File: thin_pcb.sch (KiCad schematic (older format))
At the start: 127 parts, among them J01 Conn_01x02, J02 Conn_01x02, J04 Conn_01x02, J06 Conn_01x02, J07 Conn_01x02, J08 Conn_01x02, J1 USB_B_Micro, J11 Conn_01x03, J12 Conn_01x03, J13 Conn_01x03, J14 Conn_01x03, J15 Conn_01x03, J16 Conn_01x03, J17 Conn_01x03, J18 Conn_01x03, J2 AudioJack4_Ground, J21 Conn_01x07, J22 Conn_01x07, J23 Conn_01x07, J24 Conn_01x07, J25 Conn_01x07, J26 Conn_01x07, J27 Conn_01x07, J28 Conn_01x07, J3 AudioJack4_Ground, J31 Conn_01x07, J32 Conn_01x07, J33 Conn_01x07, J34 Conn_01x07, J35 Conn_01x07, J36 Conn_01x07, J37 Conn_01x07, J38 Conn_01x07, J4 Conn_01x06, J41 Conn_01x04, J42 Conn_01x04, J43 Conn_01x04, J44 Conn_01x04, J45 Conn_01x04, J46 Conn_01x04, J47 Conn_01x04, J48 Conn_01x04, J5 Conn_01x06, J51 Conn_01x01, J52 Conn_01x01, J53 Conn_01x01, J54 Conn_01x01, J55 Conn_01x01, J56 Conn_01x01, J57 Conn_01x01, J58 Conn_01x01, J6 Conn_02x02, J7 Conn_01x02, SW11 SW_Push, SW12 SW_Push, SW13 SW_Push, SW14 SW_Push, SW15 SW_Push, SW21 SW_Push, SW22 SW_Push, SW23 SW_Push, SW24 SW_Push, SW25 SW_Push, SW252 SW_Push, SW31 SW_Push, SW32 SW_Push, SW33 SW_Push, SW34 SW_Push, SW35 SW_Push, SW41 SW_Push, SW42 SW_Push, SW422 SW_Push, SW43 SW_Push, SW44 SW_Push, SW45 SW_Push, SW452 SW_Push, SW51 SW_Push, SW52 SW_Push, SW522 SW_Push, SW53 SW_Push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

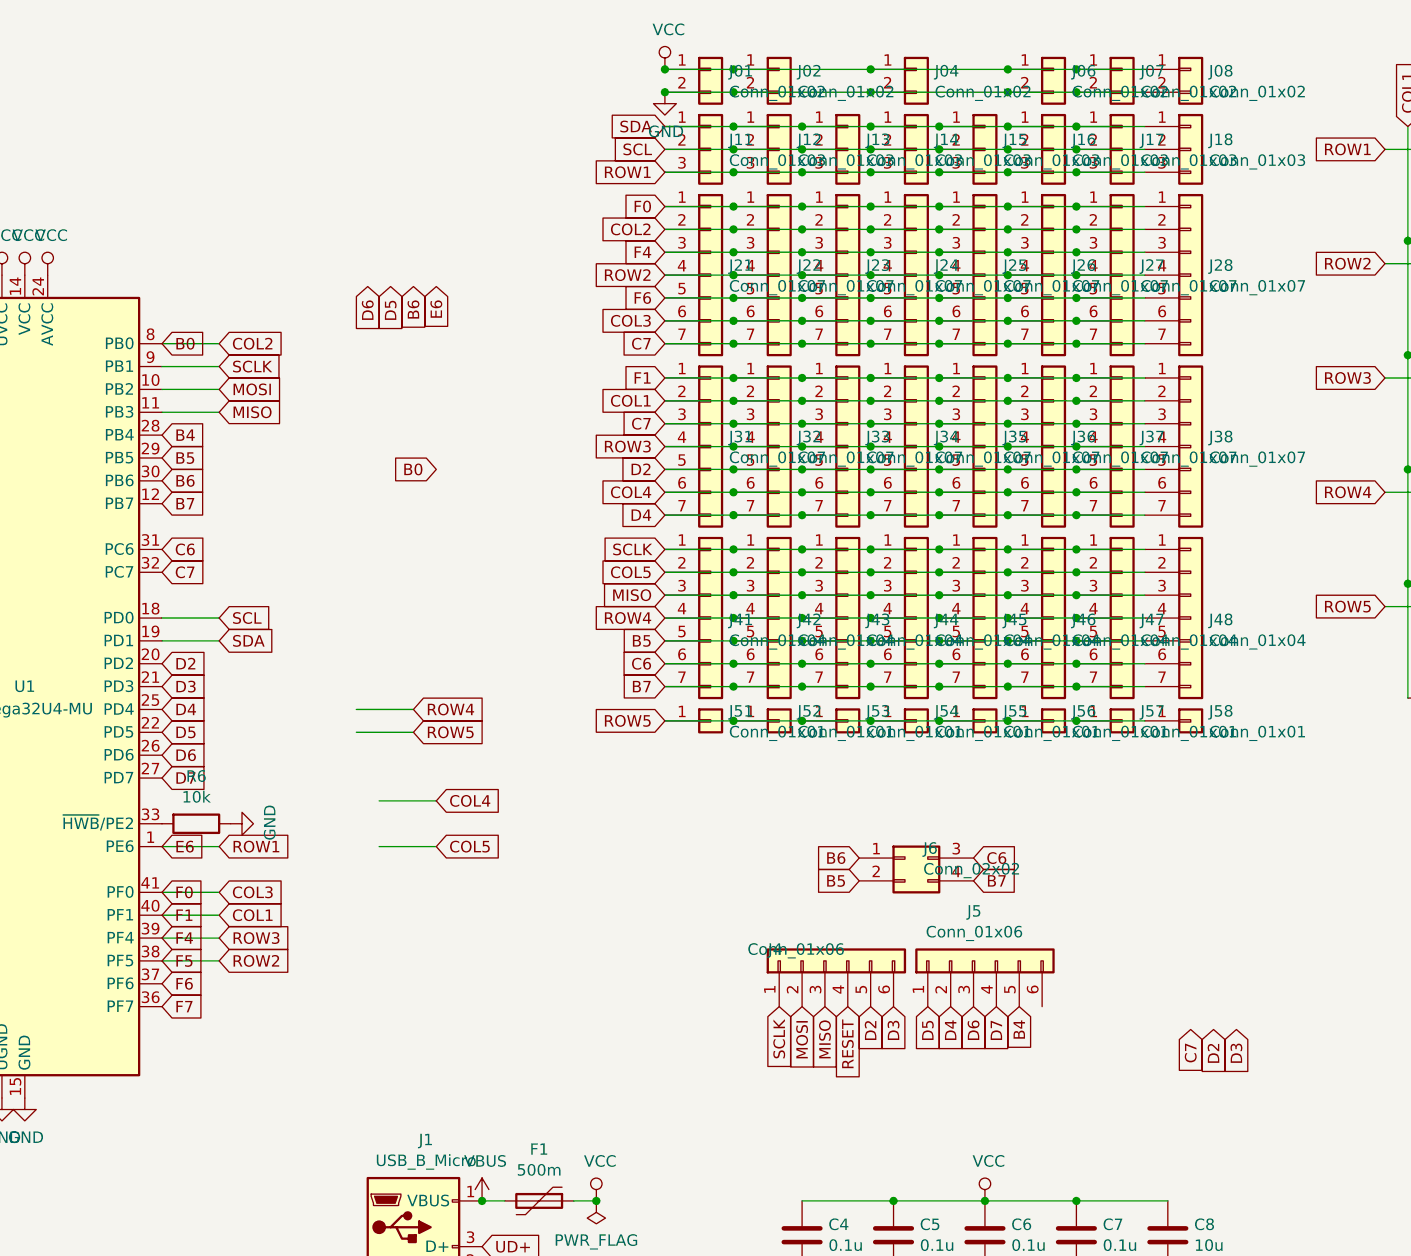
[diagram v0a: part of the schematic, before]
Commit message: draft
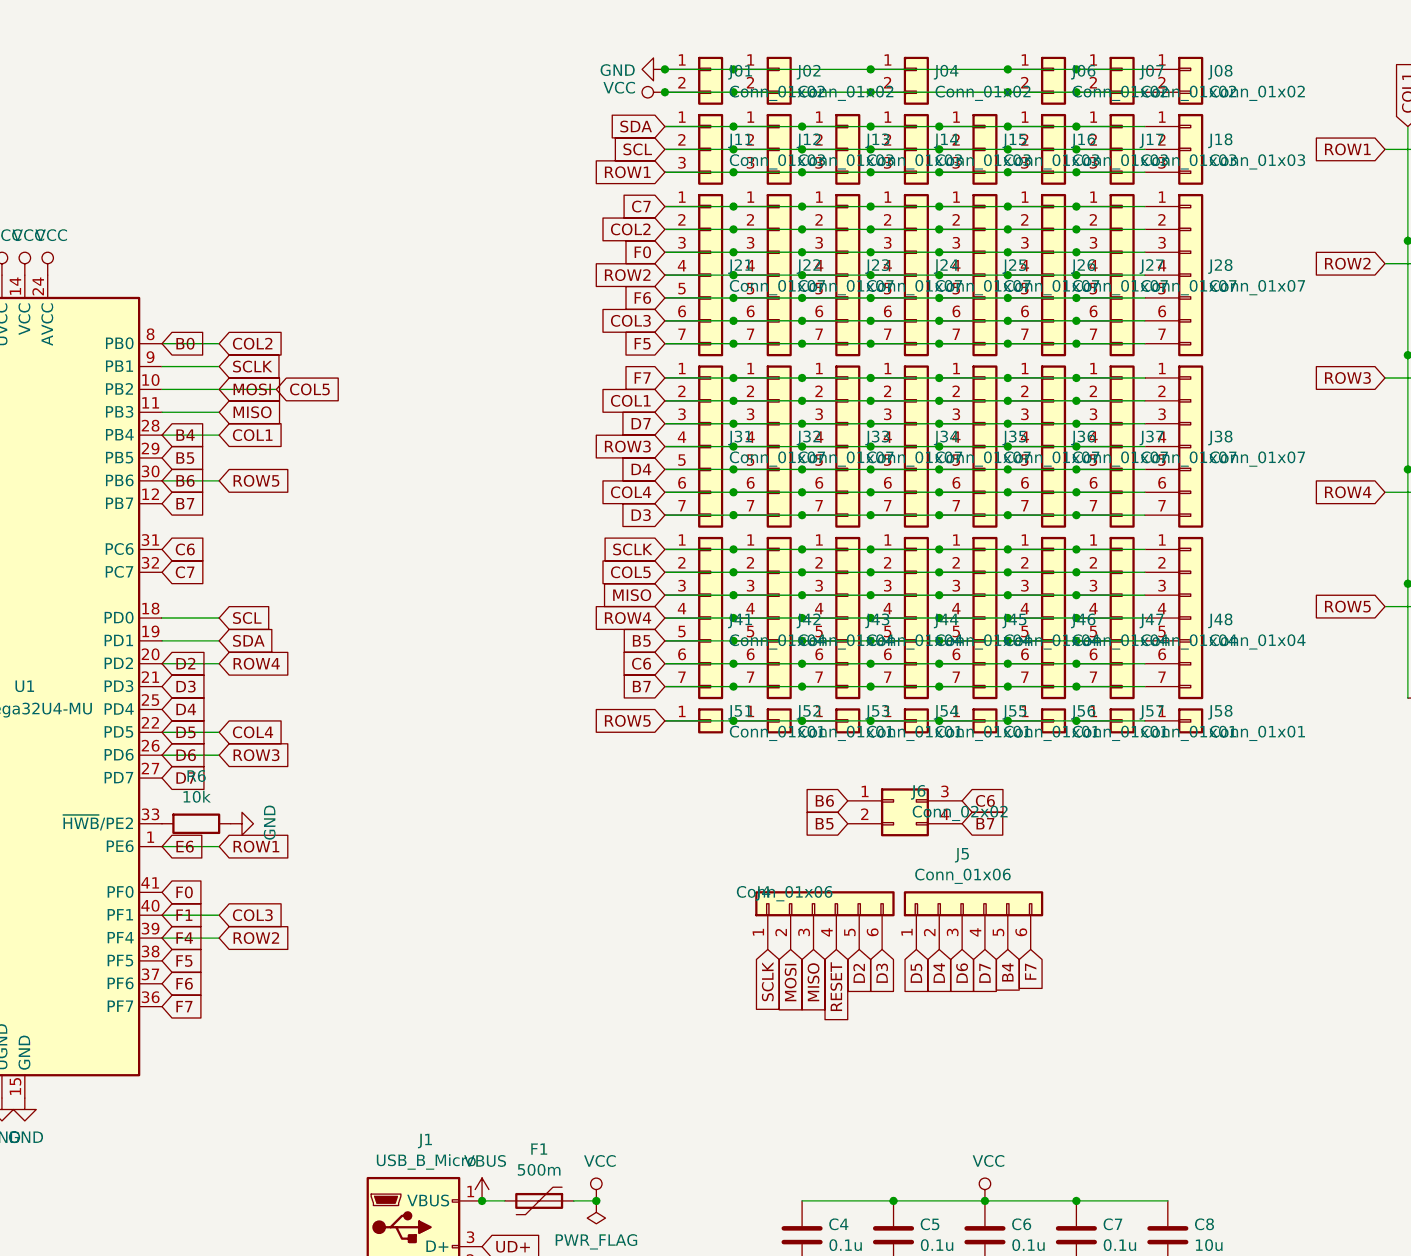
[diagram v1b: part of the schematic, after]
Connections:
- wire segments 289 -> 288
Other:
- moved on the sheet: J4, J5, J6
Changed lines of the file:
@@
 Text GLabel 9050 5700 2    50   Input ~ 0
 SCL
-Text GLabel 5150 4800 3    50   Input ~ 0
+Text GLabel 5100 4550 3    50   Input ~ 0
 MISO
-Text GLabel 5050 4800 3    50   Input ~ 0
+Text GLabel 5000 4550 3    50   Input ~ 0
 MOSI
-Text GLabel 4950 4800 3    50   Input ~ 0
+Text GLabel 4900 4550 3    50   Input ~ 0
 SCLK
-Text GLabel 5250 4800 3    50   Input ~ 0
+Text GLabel 5200 4550 3    50   Input ~ 0
 RESET
 $Comp
@@
 	0    -1   -1   0
 $EndComp
-Text GLabel 2500 4400 2    50   Input ~ 0
+Text GLabel 2500 2300 2    50   Input ~ 0
 COL1
 Text GLabel 2500 1900 2    50   Input ~ 0
 COL2
-Text GLabel 2500 4300 2    50   Input ~ 0
+Text GLabel 2500 4400 2    50   Input ~ 0
 COL3
-Text GLabel 3450 3900 2    50   Input ~ 0
+Text GLabel 2500 3600 2    50   Input ~ 0
 COL4
-Text GLabel 3450 4100 2    50   Input ~ 0
+Text GLabel 2750 2100 2    50   Input ~ 0
 COL5
 Text GLabel 2500 4100 2    50   Input ~ 0
 ROW1
-Text GLabel 2500 4600 2    50   Input ~ 0
+Text GLabel 2500 4500 2    50   Input ~ 0
 ROW2
-Text GLabel 2500 4500 2    50   Input ~ 0
+Text GLabel 2500 3700 2    50   Input ~ 0
 ROW3
-Text GLabel 3350 3500 2    50   Input ~ 0
+Text GLabel 2500 3300 2    50   Input ~ 0
 ROW4
-Text GLabel 3350 3600 2    50   Input ~ 0
+Text GLabel 2500 2500 2    50   Input ~ 0
 ROW5
 Text GLabel 2250 1900 2    50   Input ~ 0
@@
 	2250 1900 2500 1900
 Wire Wire Line
-	2250 4300 2500 4300
-Wire Wire Line
-	3200 3900 3450 3900
+	2250 2300 2500 2300
+Wire Wire Line
+	2250 3600 2500 3600
 Text GLabel 2250 3400 2    50   Input ~ 0
 D3
@@
 F7
 Wire Wire Line
-	3200 4100 3450 4100
-Wire Wire Line
 	2250 4100 2500 4100
 Wire Wire Line
-	2250 4600 2500 4600
-Wire Wire Line
 	2250 4500 2500 4500
 Wire Wire Line
-	3100 3500 3350 3500
-Wire Wire Line
-	3100 3600 3350 3600
-Text GLabel 3450 1650 3    50   Input ~ 0
-E6
+	2250 3700 2500 3700
+Wire Wire Line
+	2250 3300 2500 3300
+Wire Wire Line
+	2250 2500 2500 2500
 $Comp
 L power:VBUS #PWR0107
@@
 Wire Wire Line
 	2500 2000 2250 2000
-Wire Wire Line
-	2500 2100 2250 2100
 Wire Wire Line
 	2500 2200 2250 2200
@@
 L Connector_Generic:Conn_02x02_Top_Bottom J6
 U 1 1 5D135711
-P 5500 4150
-F 0 "J6" H 5580 4192 50  0000 L CNN
-F 1 "Conn_02x02" H 5580 4101 50  0000 L CNN
-F 2 "Connector_PinSocket_2.54mm:PinSocket_2x02_P2.54mm_Vertical" H 5500 4150 50  0001 C CNN
-F 3 "~" H 5500 4150 50  0001 C CNN
-	1    5500 4150
+P 5450 3900
+F 0 "J6" H 5530 3942 50  0000 L CNN
+F 1 "Conn_02x02" H 5530 3851 50  0000 L CNN
+F 2 "Connector_PinSocket_2.54mm:PinSocket_2x02_P2.54mm_Vertical" H 5450 3900 50  0001 C CNN
+F 3 "~" H 5450 3900 50  0001 C CNN
+	1    5450 3900
 	1    0    0    -1
 $EndComp
@@
 L Connector_Generic:Conn_01x06 J4
 U 1 1 5D135878
-P 5150 4600
-F 0 "J4" V 5200 4817 50  0000 C CNN
-F 1 "Conn_01x06" V 5200 4726 50  0000 C CNN
-F 2 "Connector_PinSocket_2.54mm:PinSocket_1x06_P2.54mm_Vertical" H 5150 4600 50  0001 C CNN
-F 3 "~" H 5150 4600 50  0001 C CNN
-	1    5150 4600
+P 5100 4350
+F 0 "J4" V 5150 4567 50  0000 C CNN
+F 1 "Conn_01x06" V 5150 4476 50  0000 C CNN
+F 2 "Connector_PinSocket_2.54mm:PinSocket_1x06_P2.54mm_Vertical" H 5100 4350 50  0001 C CNN
+F 3 "~" H 5100 4350 50  0001 C CNN
+	1    5100 4350
 	0    -1   -1   0
 $EndComp
@@
 L Connector_Generic:Conn_01x06 J5
 U 1 1 5D141D0D
-P 5800 4600
-F 0 "J5" V 6017 4596 50  0000 C CNN
-F 1 "Conn_01x06" V 5926 4596 50  0000 C CNN
-F 2 "Connector_PinSocket_2.54mm:PinSocket_1x06_P2.54mm_Vertical" H 5800 4600 50  0001 C CNN
-F 3 "~" H 5800 4600 50  0001 C CNN
-	1    5800 4600
-	0    -1   -1   0
-$EndComp
-Text GLabel 3150 1650 3    50   Input ~ 0
-D6
-Text GLabel 3250 1650 3    50   Input ~ 0
-D5
-Text GLabel 3350 1650 3    50   Input ~ 0
-B6
+P 5750 4350
+F 0 "J5" V 5967 4346 50  0000 C CNN
+F 1 "Conn_01x06" V 5876 4346 50  0000 C CNN
+F 2 "Connector_PinSocket_2.54mm:PinSocket_1x06_P2.54mm_Vertical" H 5750 4350 50  0001 C CNN
+F 3 "~" H 5750 4350 50  0001 C CNN
+	1    5750 4350
+	0    -1   -1   0
+$EndComp
 Text GLabel 4450 3400 0    50   Input ~ 0
 B7
 Text GLabel 4450 3300 0    50   Input ~ 0
 C6
-Text GLabel 6750 4900 3    50   Input ~ 0
-C7
-Text GLabel 6850 4900 3    50   Input ~ 0
-D2
-Text GLabel 6950 4900 3    50   Input ~ 0
-D3
-Text GLabel 5700 4800 3    50   Input ~ 0
+Text GLabel 5650 4550 3    50   Input ~ 0
 D4
 $Comp
@@
 	1    0    0    -1
 $EndComp
-Text GLabel 3450 2450 0    50   Input ~ 0
-B0
-Text GLabel 4450 2250 0    50   Input ~ 0
-C7
-Text GLabel 4450 2450 0    50   Input ~ 0
-D2
-Text GLabel 4450 2650 0    50   Input ~ 0
-D4
-Text GLabel 4450 1500 0    50   Input ~ 0
-F4
 $Comp
 L Connector_Generic:Conn_01x07 J21
@@
 Text GLabel 4450 2900 0    50   Input ~ 0
 COL5
-Text GLabel 4450 2050 0    50   Input ~ 0
-F1
 Connection ~ 7700 1450
 Connection ~ 8000 1050
@@
 Wire Wire Line
 	9800 1450 9800 1950
-Text GLabel 6000 4800 3    50   Input ~ 0
+Text GLabel 5950 4550 3    50   Input ~ 0
 B4
 Text GLabel 4450 3200 0    50   Input ~ 0
 B5
-Text GLabel 4450 1300 0    50   Input ~ 0
+Text GLabel 4450 1500 0    50   Input ~ 0
 F0
 Text GLabel 4450 1700 0    50   Input ~ 0
 F6
-Text GLabel 4450 1900 0    50   Input ~ 0
+Text GLabel 4450 1300 0    50   Input ~ 0
 C7
 Text GLabel 4450 950  0    50   Input ~ 0
@@
 L power:GND #PWR0115
 U 1 1 5D30B159
+P 4450 700
+F 0 "#PWR0115" H 4450 450 50  0001 C CNN
+F 1 "GND" V 4455 572 50  0000 R CNN
+F 2 "" H 4450 700 50  0001 C CNN
+F 3 "" H 4450 700 50  0001 C CNN
+	1    4450 700
+	0    1    1    0
+$EndComp
+$Comp
+L power:VCC #PWR0116
+U 1 1 5D30B28B
 P 4450 800
-F 0 "#PWR0115" H 4450 550 50  0001 C CNN
-F 1 "GND" H 4455 627 50  0000 C CNN
+F 0 "#PWR0116" H 4450 650 50  0001 C CNN
+F 1 "VCC" V 4468 927 50  0000 L CNN
 F 2 "" H 4450 800 50  0001 C CNN
 F 3 "" H 4450 800 50  0001 C CNN
 	1    4450 800
-	1    0    0    -1
-$EndComp
-$Comp
-L power:VCC #PWR0116
-U 1 1 5D30B28B
-P 4450 700
-F 0 "#PWR0116" H 4450 550 50  0001 C CNN
-F 1 "VCC" H 4467 873 50  0000 C CNN
-F 2 "" H 4450 700 50  0001 C CNN
-F 3 "" H 4450 700 50  0001 C CNN
-	1    4450 700
-	1    0    0    -1
+	0    -1   -1   0
 $EndComp
 $Comp
@@
 Wire Wire Line
 	6550 700  6250 700
-Connection ~ 4450 700
 Connection ~ 4750 700
 Wire Wire Line
@@
 Wire Wire Line
 	6550 800  6250 800
-Connection ~ 4450 800
 Connection ~ 4750 800
 Wire Wire Line
@@
 Wire Wire Line
 	6250 3400 5950 3400
-Text GLabel 5800 4250 2    50   Input ~ 0
+Text GLabel 5750 4000 2    50   Input ~ 0
 B7
-Text GLabel 5800 4150 2    50   Input ~ 0
+Text GLabel 5750 3900 2    50   Input ~ 0
 C6
-Text GLabel 5300 4250 0    50   Input ~ 0
+Text GLabel 5250 4000 0    50   Input ~ 0
 B5
 Connection ~ 5950 700
@@
 Wire Wire Line
 	5350 800  5950 800
-Text GLabel 5350 4800 3    50   Input ~ 0
+Text GLabel 5300 4550 3    50   Input ~ 0
 D2
-Text GLabel 5450 4800 3    50   Input ~ 0
+Text GLabel 5400 4550 3    50   Input ~ 0
 D3
-Text GLabel 5600 4800 3    50   Input ~ 0
+Text GLabel 5550 4550 3    50   Input ~ 0
 D5
-Text GLabel 5800 4800 3    50   Input ~ 0
+Text GLabel 5750 4550 3    50   Input ~ 0
 D6
-Text GLabel 5900 4800 3    50   Input ~ 0
+Text GLabel 5850 4550 3    50   Input ~ 0
 D7
-Text GLabel 5300 4150 0    50   Input ~ 0
+Text GLabel 5250 3900 0    50   Input ~ 0
 B6
+Text GLabel 6050 4550 3    50   Input ~ 0
+F7
+Text GLabel 4450 1900 0    50   Input ~ 0
+F5
+Text GLabel 4450 2450 0    50   Input ~ 0
+D4
+Text GLabel 4450 2250 0    50   Input ~ 0
+D7
+Text GLabel 4450 2050 0    50   Input ~ 0
+F7
+Text GLabel 4450 2650 0    50   Input ~ 0
+D3
+Wire Wire Line
+	2250 2100 2750 2100
+Connection ~ 4450 800
+Connection ~ 4450 700
 $EndSCHEMATC

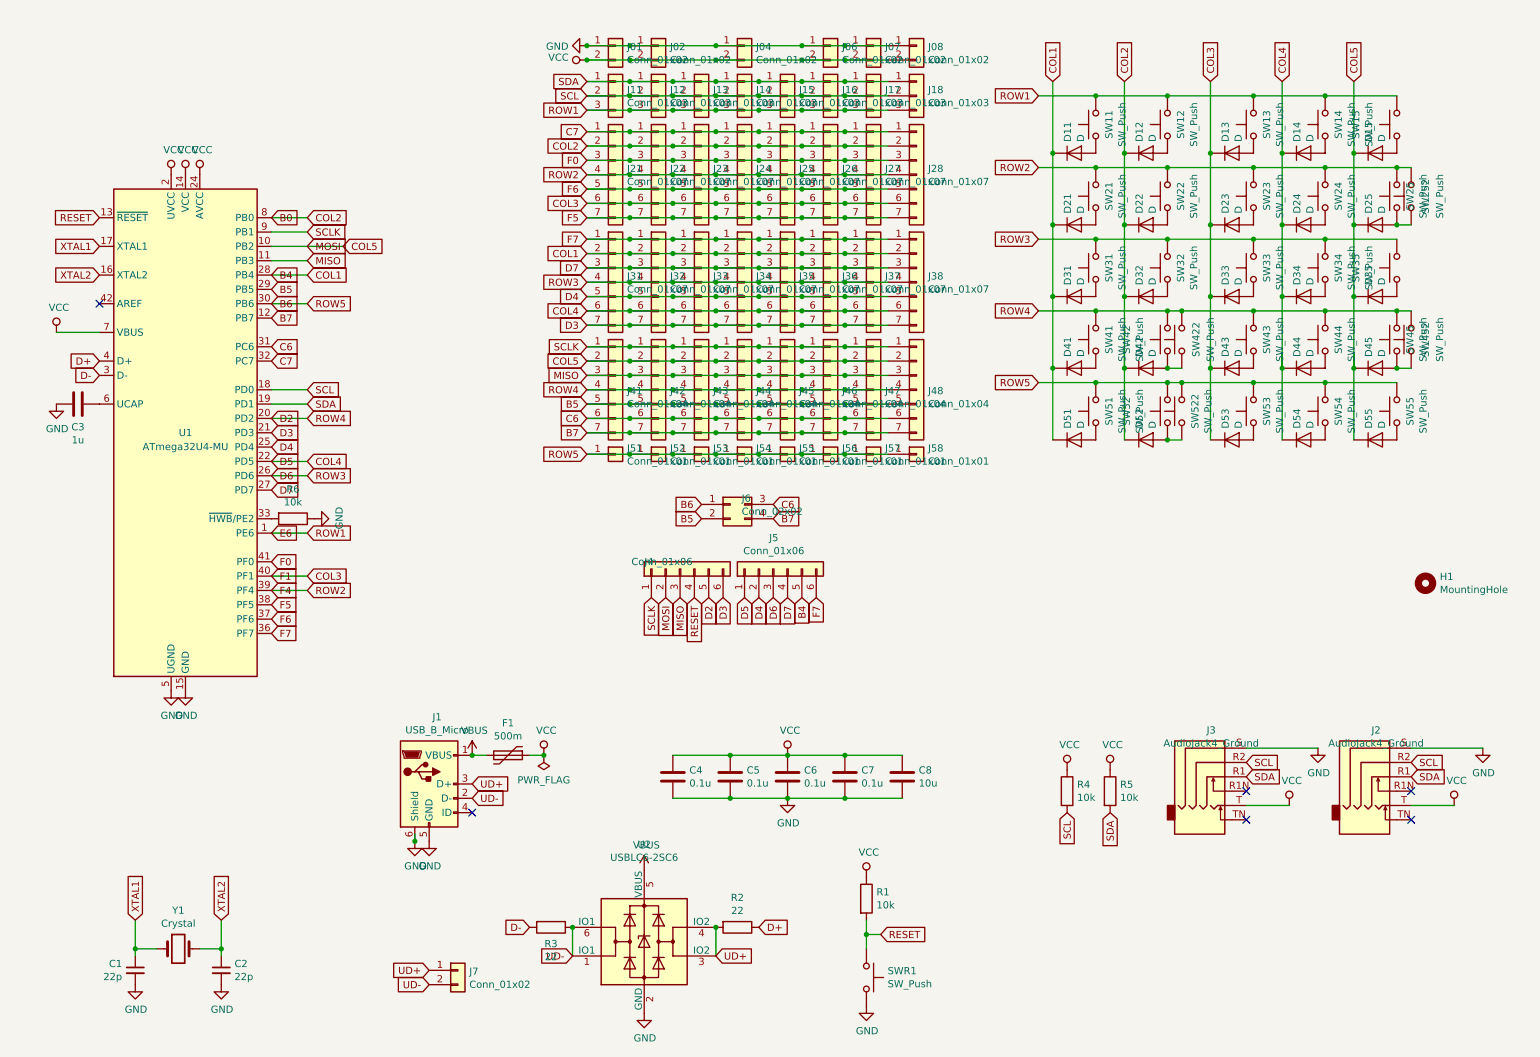
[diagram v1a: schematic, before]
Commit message: arrange schema
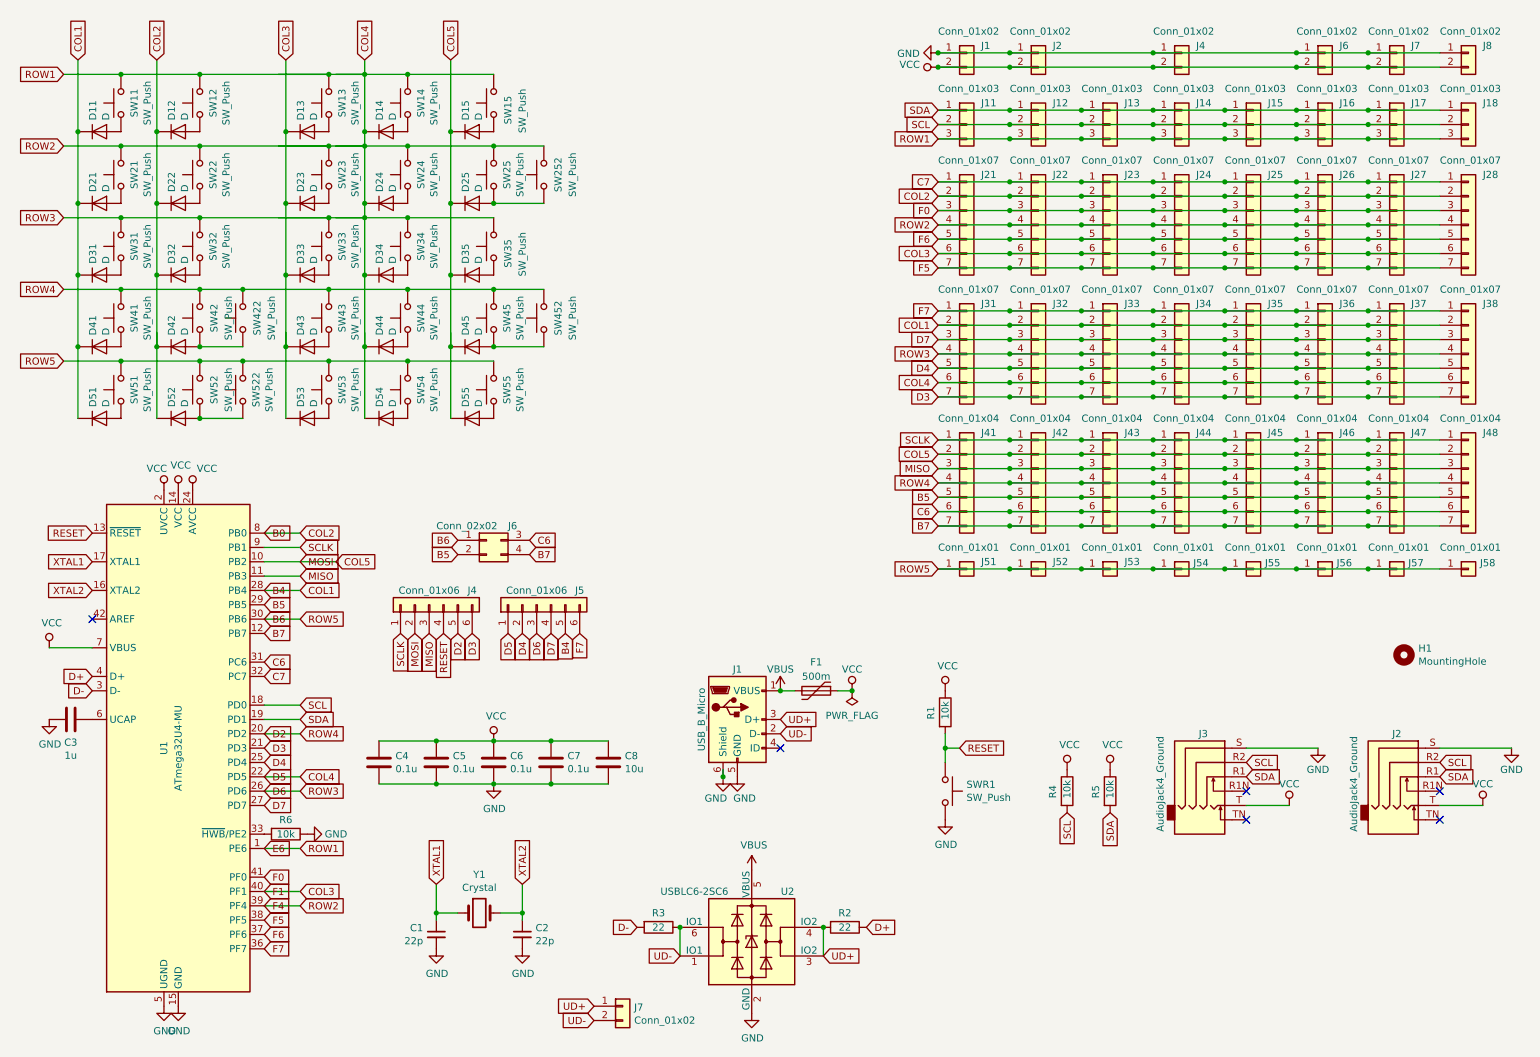
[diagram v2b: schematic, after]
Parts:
- renumbered J01 to J1, J02 to J2, J04 to J4, J06 to J6, J07 to J7, J08 to J8
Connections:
- wire segments 288 -> 300
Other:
- moved on the sheet: C1, C2, C3, C4, C5, C6, C7, C8, D11, D12, D13, D14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
